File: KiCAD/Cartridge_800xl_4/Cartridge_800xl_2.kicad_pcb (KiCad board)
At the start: 4 copper layers, 64 x 80.2 mm, 21 parts, among them SW1 Reset, U1 27C512, U2 74HC165, U3 74HC595, U4 GAL16V8, U5 TXS0108EPW, U6 mini_esp32

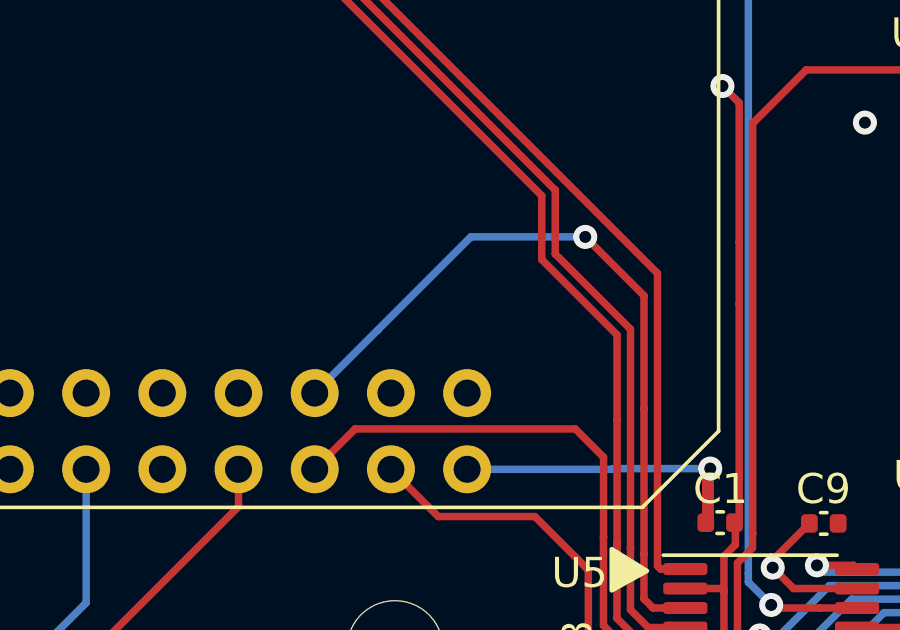
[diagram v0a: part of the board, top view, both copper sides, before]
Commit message: pcb update
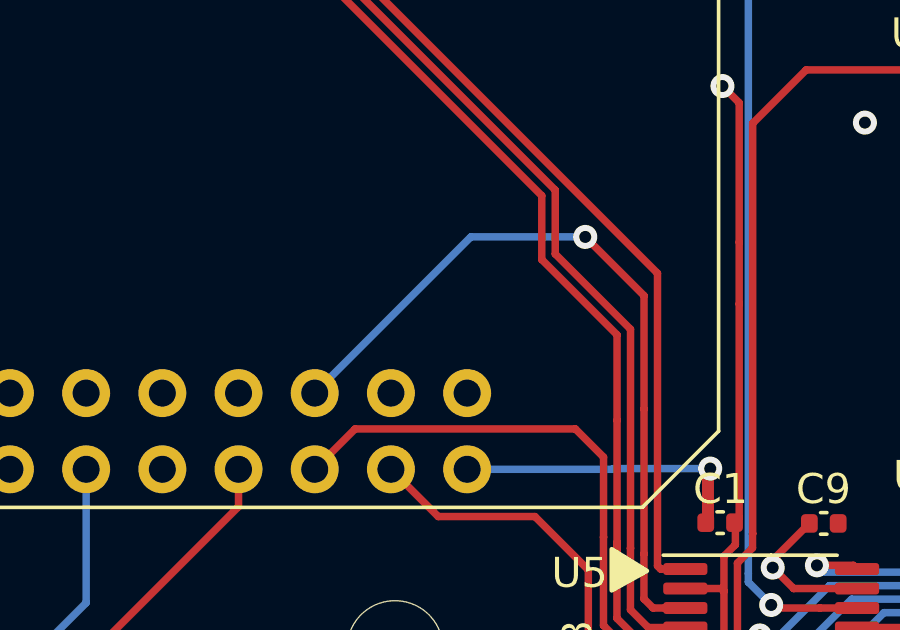
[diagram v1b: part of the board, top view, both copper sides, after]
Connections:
- U5 pad 3: iIO1 -> IO1L
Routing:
- net iIO1: track 25.6 -> 0.00 mm, vias 1 -> 0
- net IO1L: track 0.00 -> 25.6 mm, vias 0 -> 1
